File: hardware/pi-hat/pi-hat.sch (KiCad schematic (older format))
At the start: 97 parts, among them J1 PWR_IN, J10 6-8, J11 PWM0, J12 PWM1, J13 KLPX-0848A-2-B, J14 KLPX-0848A-2-R, J2 A-F, J3 40HAT, J4 G-M, J5 N-Q, J6 PANEL_PWR, J7 PANEL_CTL, J8 2-5, J9 WP, Q1 DMG2305UX, Q2 DMMT5401, Q3 DMN6075S, Q4 DMP4065S, Q5 DMN6075S, U1 CAT24C32, U10 L78L33_SOT89, U11 L78L33_SOT89, U12 PCM5122PW, U13 TSR_2-2450, U2 CM1293A, U3 CM1293A, U4 CM1293A, U5 CM1293A, U6 CM1293A, U7 CM1293A, U8 MCP23S17_SO, U9 MCP23S17_SO

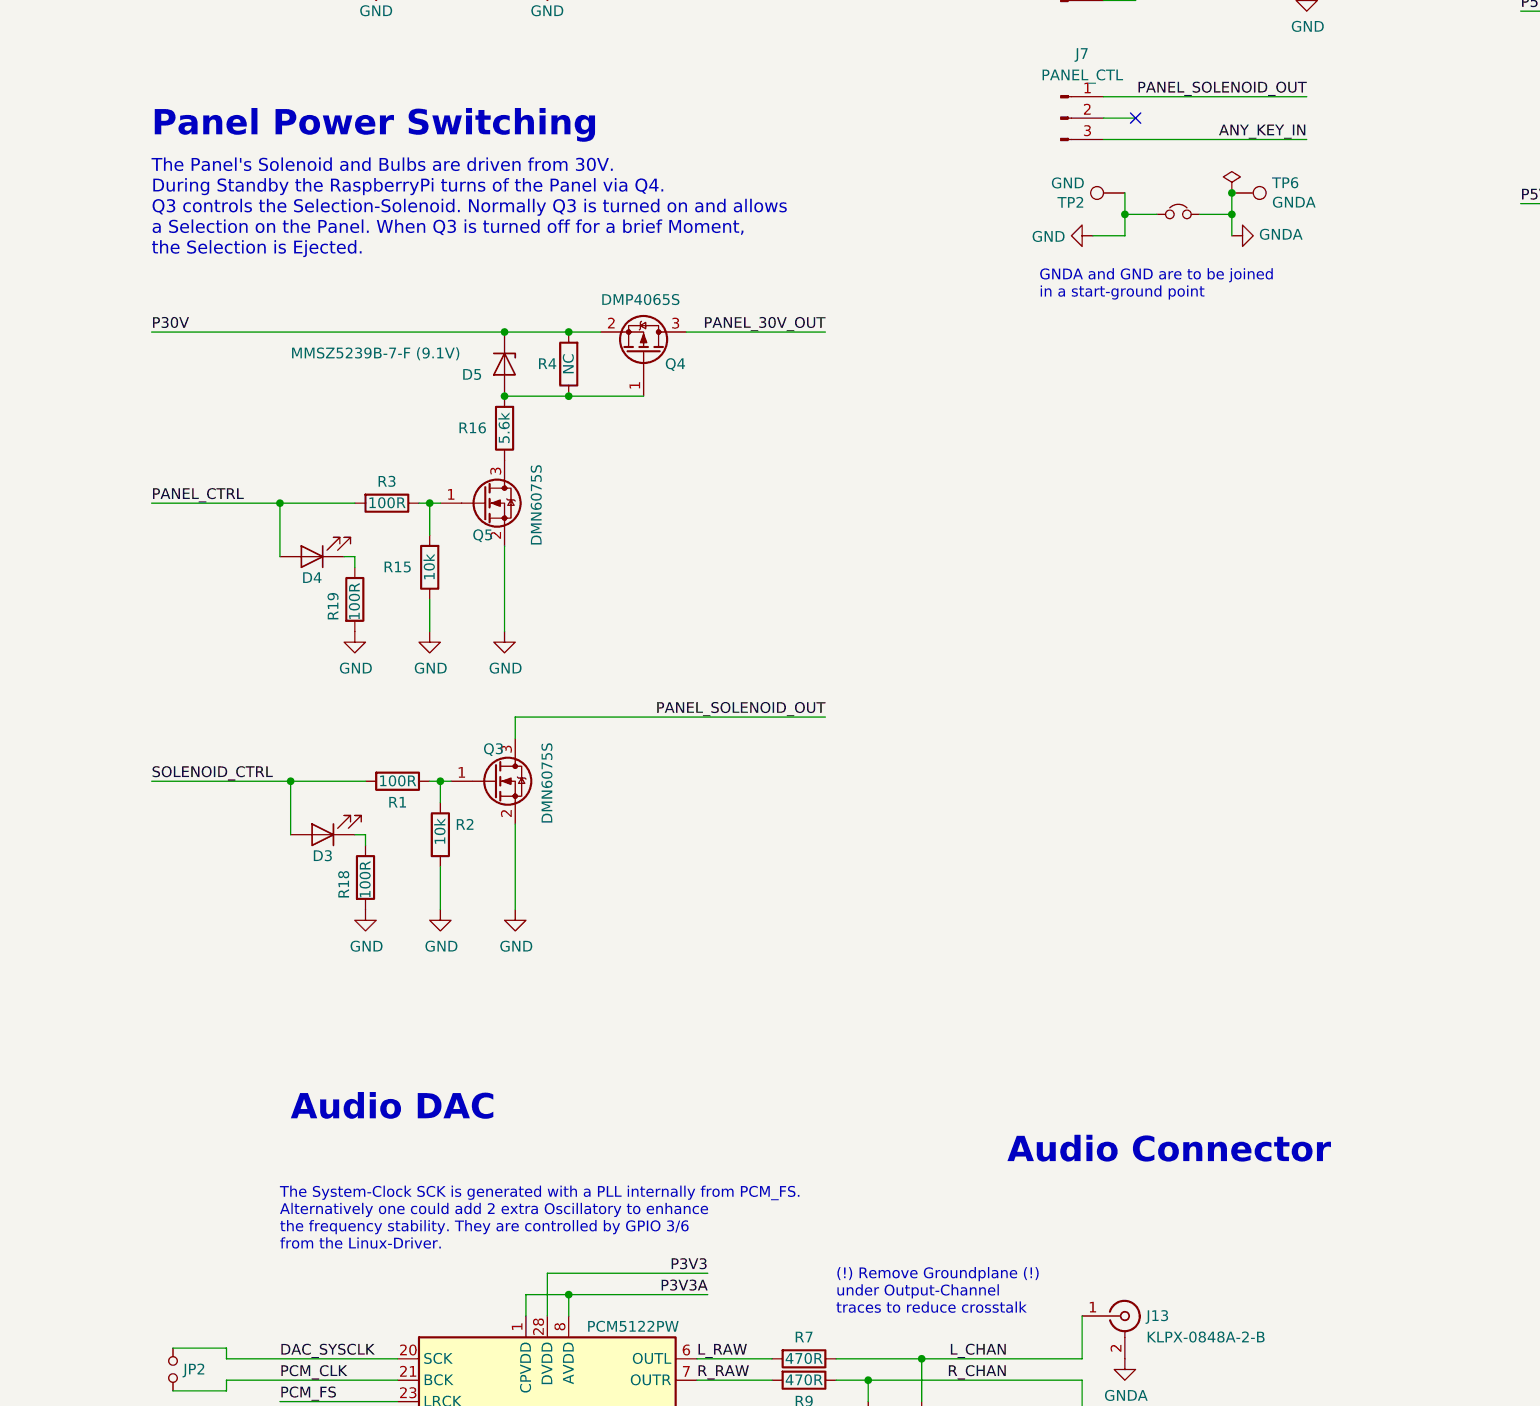
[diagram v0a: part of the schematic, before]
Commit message: documentation
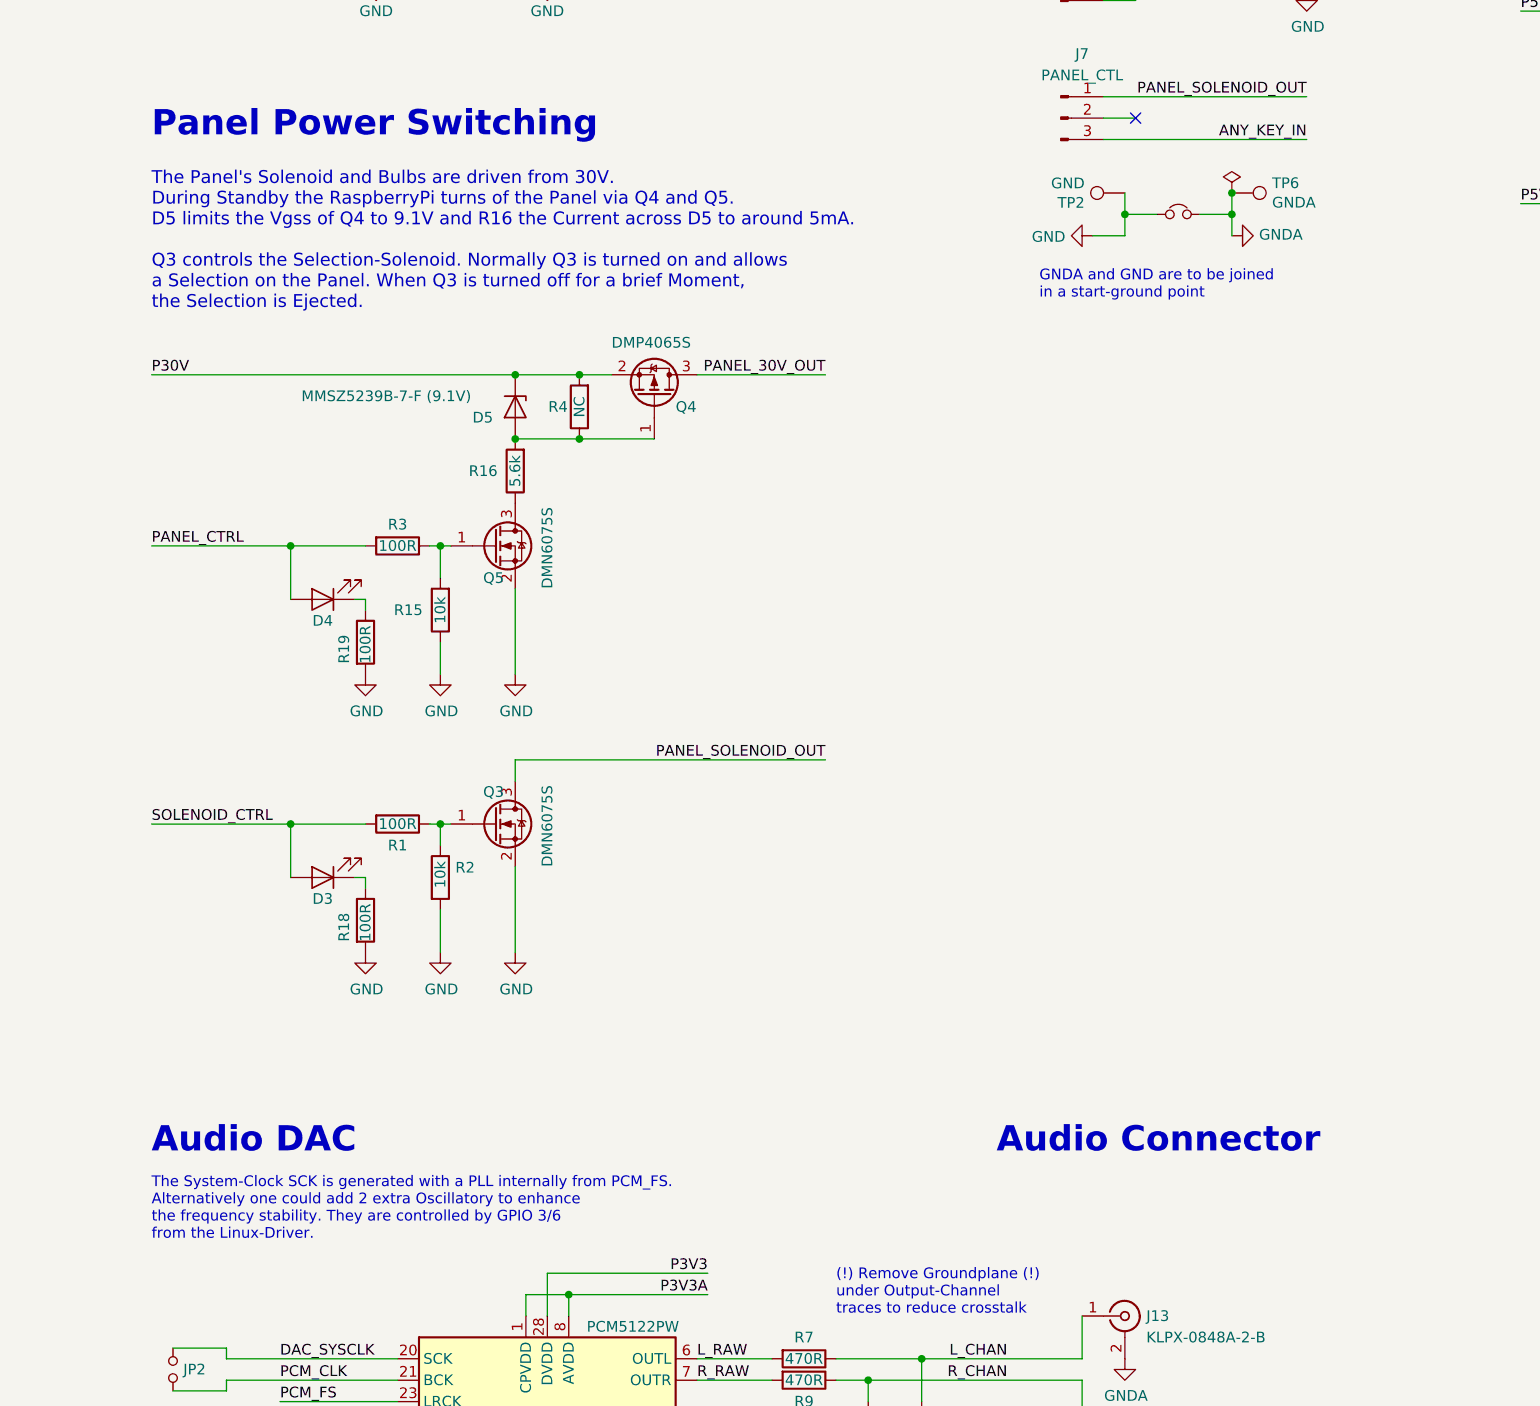
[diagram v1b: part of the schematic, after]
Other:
- note added: "The Panel's Solenoid and Bulbs are driven from 30V.\nDuring Standby the RaspberryPi turns of the Panel via Q4 and Q5.\nD5 limits the Vgss of Q4 to 9.1V and R16 the Current across D5 to around 5mA.\n\nQ3 controls the Selection-Solenoid. Normally Q3 is turned on and allows\na Selection on the Panel. When Q3 is turned off for a brief Moment,\nthe Selection is Ejected."
- note removed: "The Panel's Solenoid and Bulbs are driven from 30V.\nDuring Standby the RaspberryPi turns of the Panel via Q4.\nQ3 controls the Selection-Solenoid. Normally Q3 is turned on and allows\na Selection on the Panel. When Q3 is turned off for a brief Moment,\nthe Selection is Ejected."
- moved on the sheet: D3, D4, D5, Q3, Q4, Q5, R1, R15, R16, R18, R19, R2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
